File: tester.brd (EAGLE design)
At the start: 56 x 67 mm, 72 parts, among them IC1 ATmega8/88/168, K1 NA 05W K, M1 SP6000C-180, P1 250, P2 10k lin, Q1 BC847CSMD, Q2 BC847CSMD, Q3 BC807-40SMD, Q4 8,000 MHz, Q5 BC847CSMD, Q9 IRFR9024, U1 LT1004CZ-2.5, U2 MCP1702-5002, U3 MCP1702-5002, U4 LM339D, U5 BCR421U, X1 NEB21R

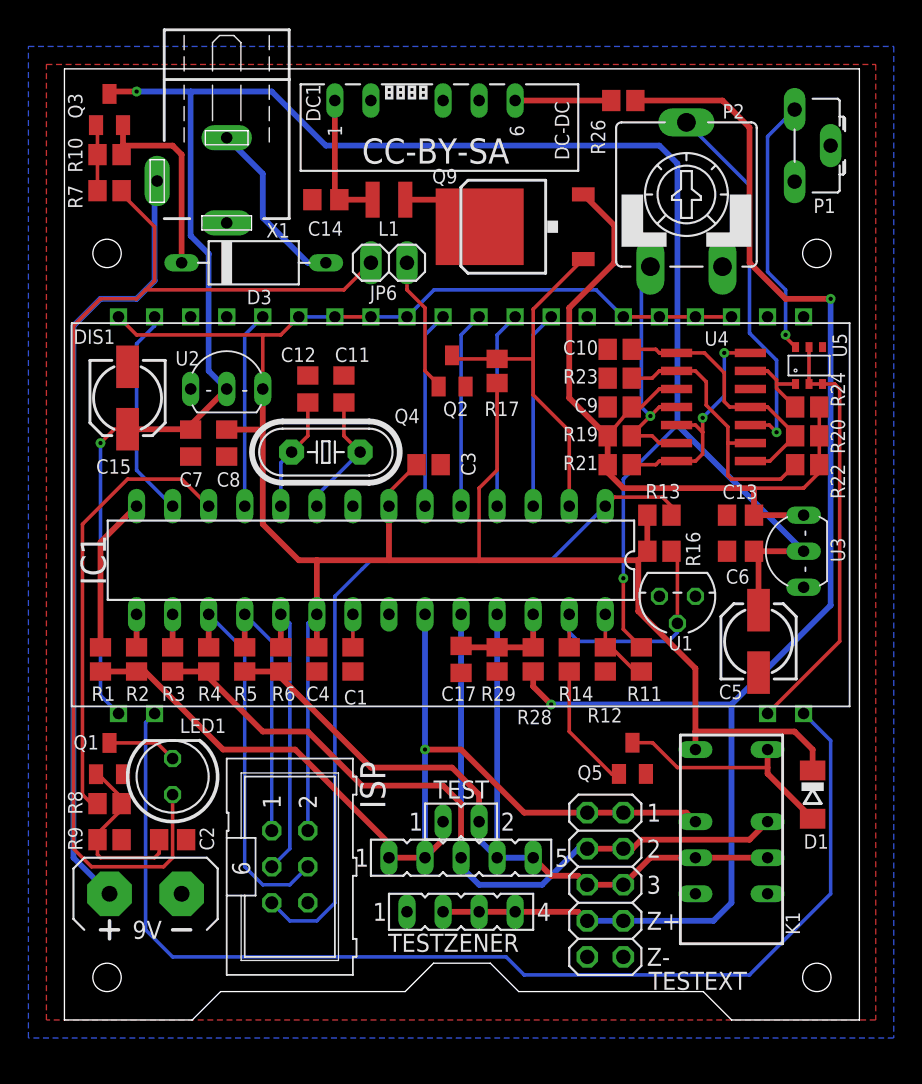
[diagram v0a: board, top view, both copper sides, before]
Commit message: some change
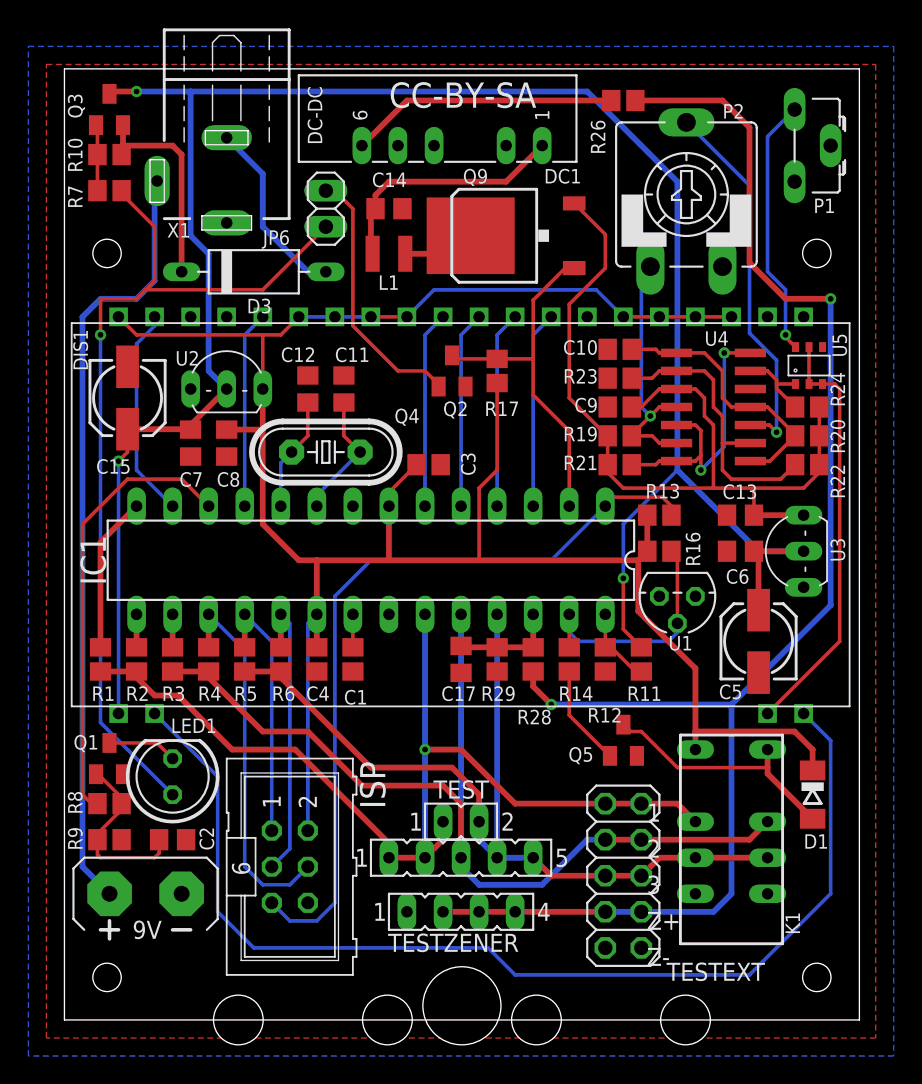
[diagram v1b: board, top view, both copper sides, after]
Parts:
- removed PLATINENSAMMLER: LP_NUMBER08_SILK_TOP, Platinensammler:LP_NUMBER_SILK_TOP
- M1: value SP6000C-180 -> SP6000H-180; device strapubox:SP-6000-C-180 -> strapubox:SP6000H-180
- moved JP6 5.85 mm to (18.4, 57.1), turned to 270 degrees
- moved C14 4.49 mm to (22.9, 57.1), turned to 0 degrees
- moved L1 3.81 mm to (22.9, 54.0)
- moved DC1 3.70 mm to (27.3, 61.6), turned to 270 degrees
- moved Q5 1.42 mm to (39.4, 19.7)
- moved JP4 1.42 mm to (39.4, 10.2)
- moved Q9 0.90 mm to (31.1, 55.2)
- moved D3 0.64 mm to (13.3, 52.7)
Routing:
- net N$21: track 80.1 -> 63.2 mm, vias 0 -> 1
- net N$28: track 6.77 -> 18.9 mm
- net N$3: track 9.64 -> 18.6 mm
- net N$25: track 9.46 -> 17.7 mm
- net +5V/2: track 55.7 -> 61.0 mm
- net N$2: track 80.9 -> 76.7 mm
- net V+: track 152.6 -> 149.0 mm
- net N$7: track 16.9 -> 20.6 mm
- net N$22: track 8.97 -> 7.14 mm
- net N$18: track 16.4 -> 17.6 mm
- net +30V: track 107.2 -> 106.3 mm
- net N$24: track 6.03 -> 5.13 mm
- net N$4: track 19.9 -> 20.6 mm
- net N$5: track 14.3 -> 15.0 mm
- net N$11: track 12.4 -> 13.1 mm
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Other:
- outline, holes or cut-outs redrawn
